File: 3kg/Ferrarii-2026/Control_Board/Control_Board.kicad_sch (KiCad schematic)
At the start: 28 parts, among them J1 Left Signal Bus, J2 Start Module, J3 Optional Back Diffusion, J4 Right Signal Bus, J5 LCD Screen, J6 Left Encoder, J7 Right Encoder, J8 Motor Control Pins, U2 1101M2S3CQE2, U3 TSR1-2450E

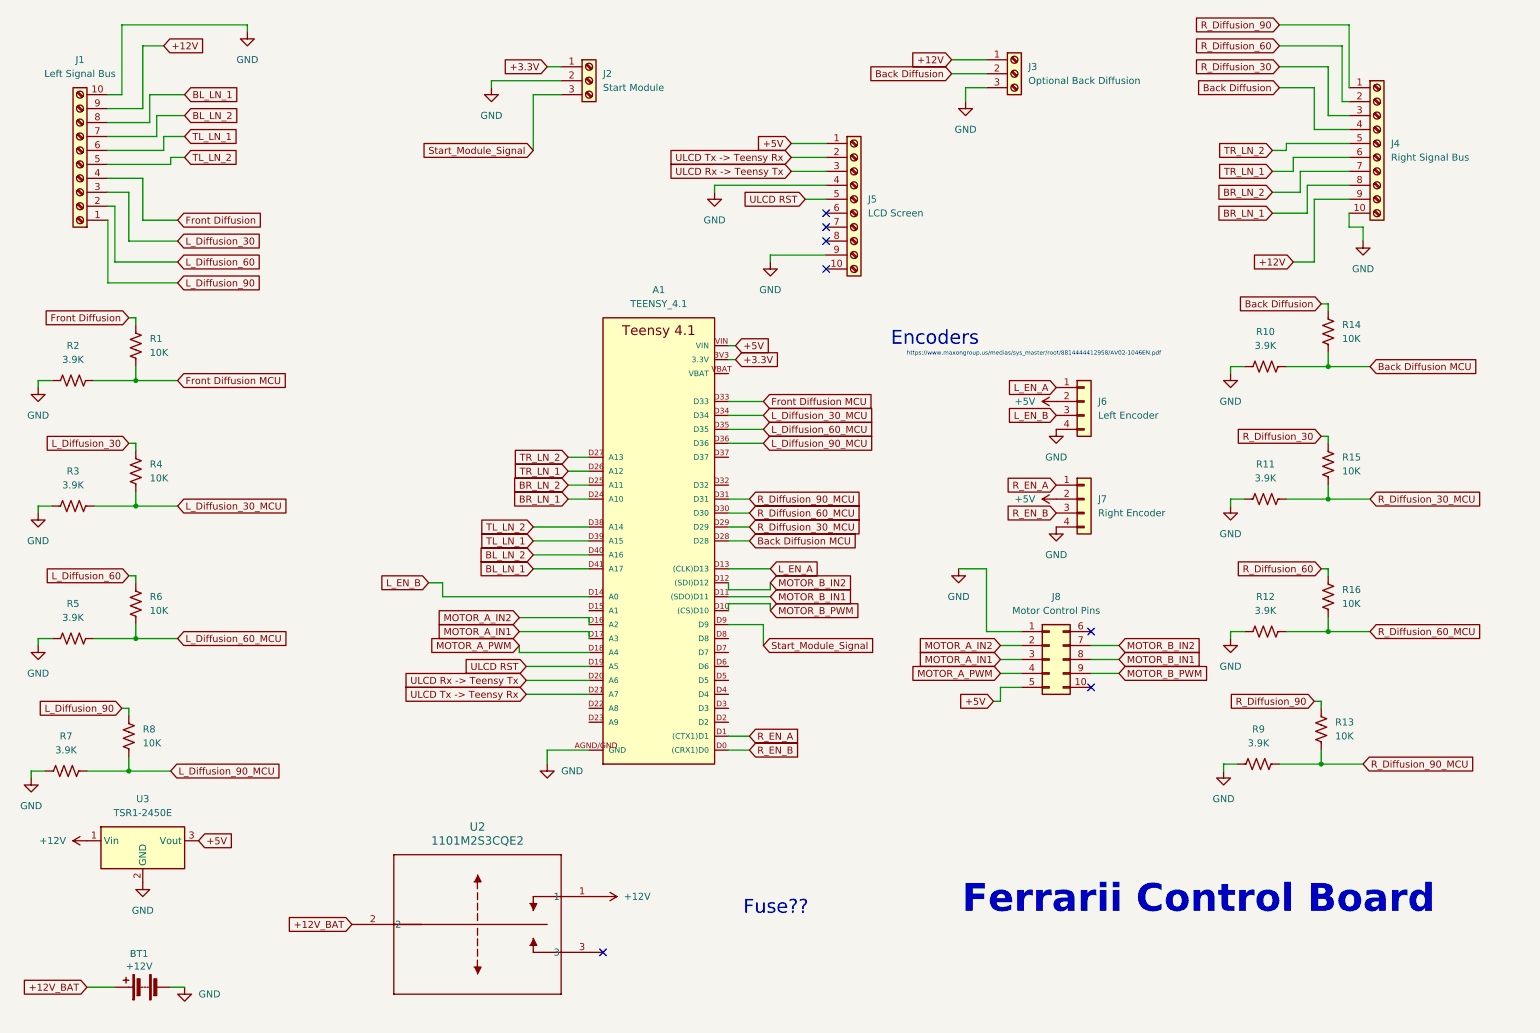
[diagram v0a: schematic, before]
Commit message: changed some things
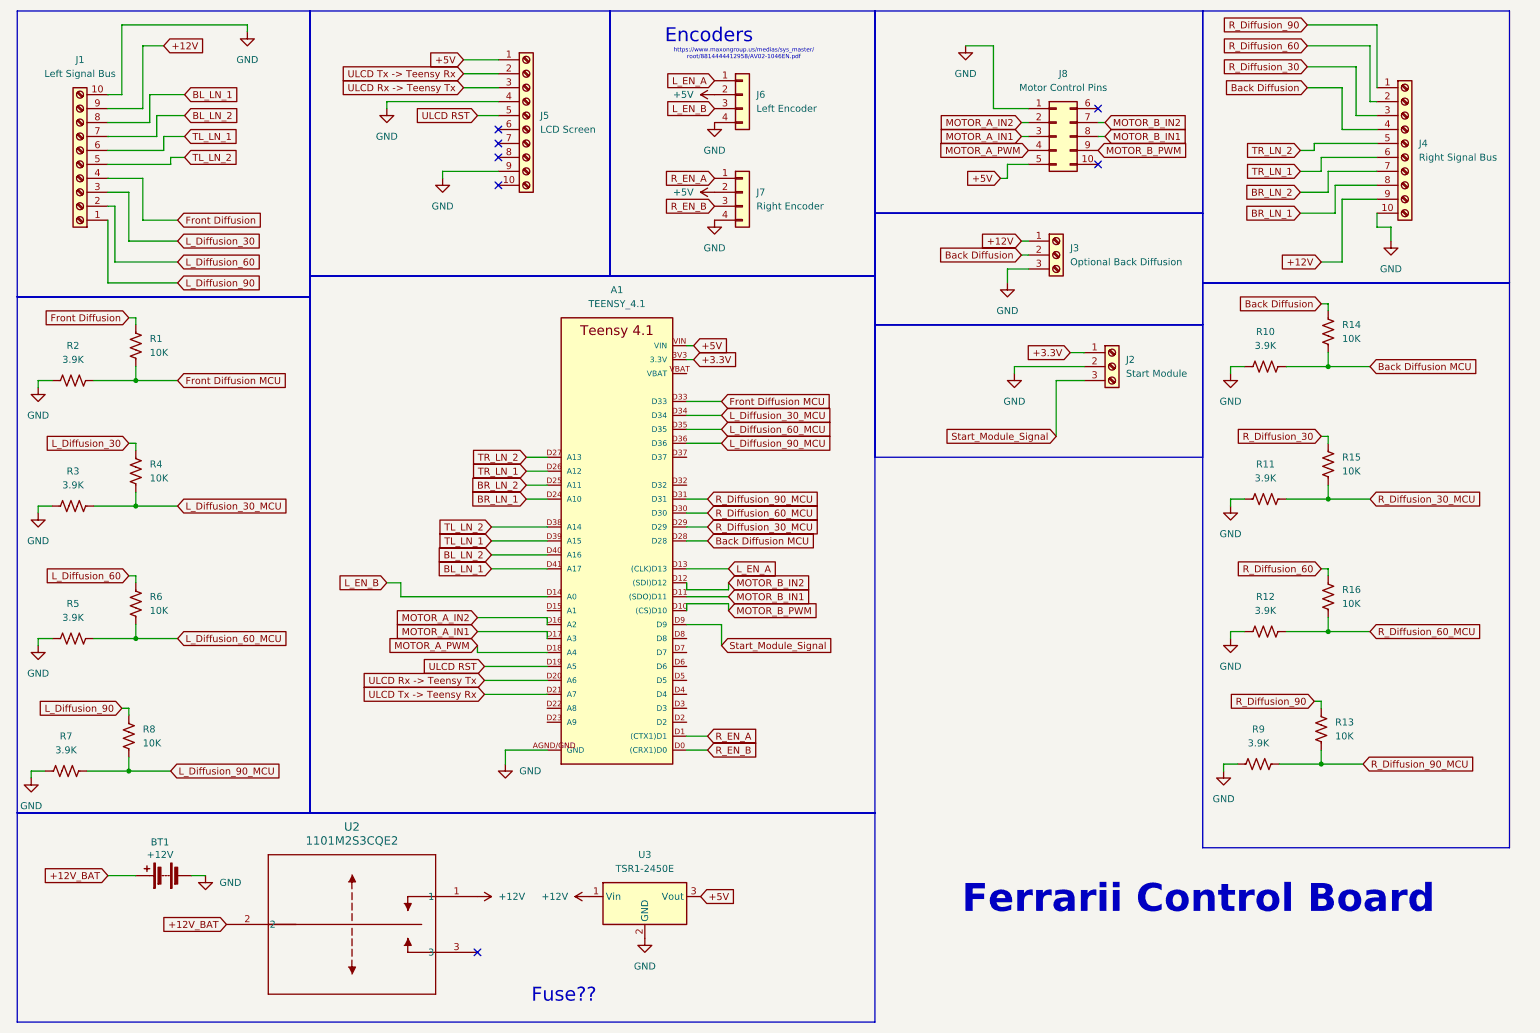
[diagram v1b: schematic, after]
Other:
- note added: "https://www.maxongroup.us/medias/sys_master/ root/8814444412958/AV02-1046EN.pdf"
- note removed: "https://www.maxongroup.us/medias/sys_master/root/8814444412958/AV02-1046EN.pdf"
- moved on the sheet: A1, BT1, J2, J3, J4, J5, J6, J7, J8, U2, U3
